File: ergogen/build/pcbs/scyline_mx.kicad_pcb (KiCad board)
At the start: 2 copper layers, 133 x 104.7 mm, 106 parts, among them J1 qwiik_jst

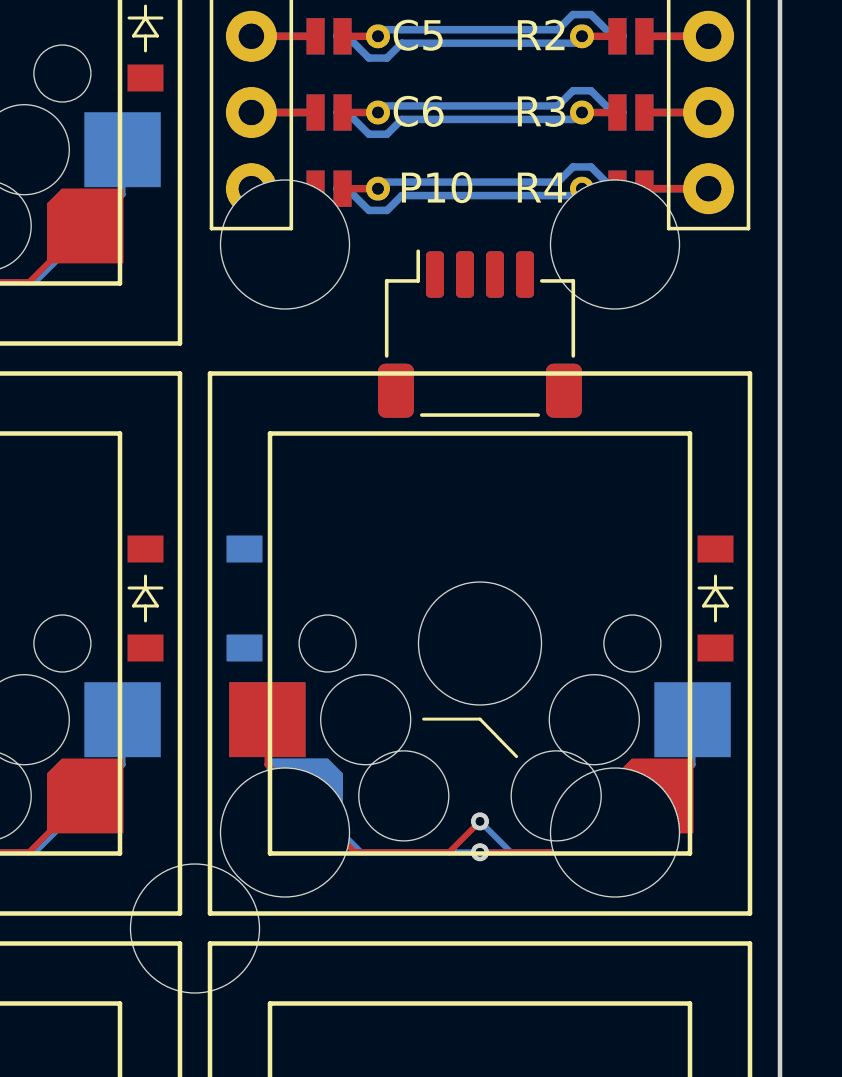
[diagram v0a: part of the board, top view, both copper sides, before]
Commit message: Build
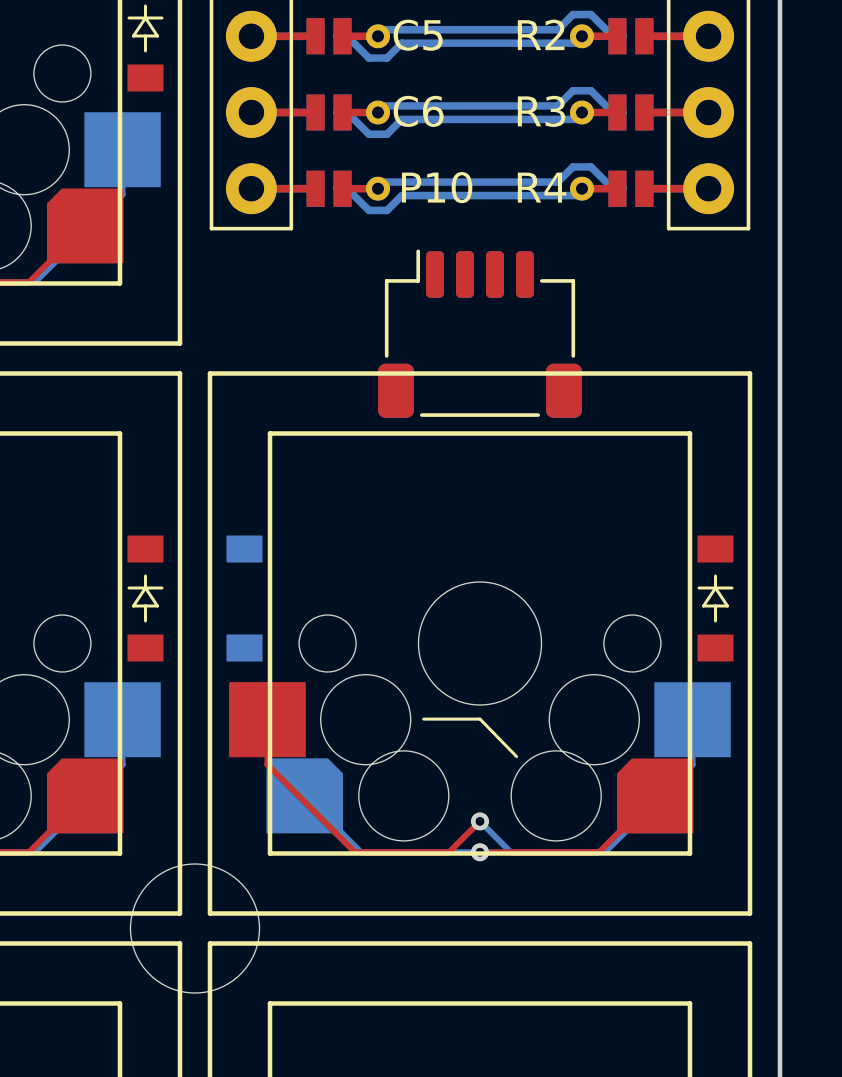
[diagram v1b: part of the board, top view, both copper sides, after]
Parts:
- removed MH10, MH11, MH12, MH13: , ceoloide:mounting_hole_npth
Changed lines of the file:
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@@
-    )
-  )
-  (footprint "ceoloide:mounting_hole_npth"
-    (layer "F.Cu")
-    (at 207.5 106.11 0)
-    (property "Reference" "MH10"
-      (at 0 2.55 0)
-      (layer "F.SilkS")
-      hide
-      (effects (font (size 1 1) (thickness 0.15)))
-    )
-    (pad "" np_thru_hole circle
-      (at 0 0 0)
-      (size 4.3 4.3)
-      (drill 4.3)
-      (layers "*.Cu" "*.Mask")
-    )
-  )
-  (footprint "ceoloide:mounting_hole_npth"
-    (layer "F.Cu")
-    (at 218.5 106.11 0)
-    (property "Reference" "MH11"
-      (at 0 2.55 0)
-      (layer "F.SilkS")
-      hide
-      (effects (font (size 1 1) (thickness 0.15)))
-    )
-    (pad "" np_thru_hole circle
-      (at 0 0 0)
-      (size 4.3 4.3)
-      (drill 4.3)
-      (layers "*.Cu" "*.Mask")
-    )
-  )
-  (footprint "ceoloide:mounting_hole_npth"
-    (layer "F.Cu")
-    (at 207.5 125.71 0)
-    (property "Reference" "MH12"
-      (at 0 2.55 0)
-      (layer "F.SilkS")
-      hide
-      (effects (font (size 1 1) (thickness 0.15)))
-    )
-    (pad "" np_thru_hole circle
-      (at 0 0 0)
-      (size 4.3 4.3)
-      (drill 4.3)
-      (layers "*.Cu" "*.Mask")
-    )
-  )
-  (footprint "ceoloide:mounting_hole_npth"
-    (layer "F.Cu")
-    (at 218.5 125.71 0)
-    (property "Reference" "MH13"
-      (at 0 2.55 0)
-      (layer "F.SilkS")
-      hide
-      (effects (font (size 1 1) (thickness 0.15)))
-    )
-    (pad "" np_thru_hole circle
-      (at 0 0 0)
-      (size 4.3 4.3)
-      (drill 4.3)
-      (layers "*.Cu" "*.Mask")
     )
   )
